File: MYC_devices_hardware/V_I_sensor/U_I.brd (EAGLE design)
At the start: 75.5 x 39.7 mm, 35 parts, among them IC2 MEGA8-AI, IC3 78L05, IC4 MAX3232CSE, Q1 20MH2, U1 INA219AIDCNR, X1 8-15V, X4 RS232

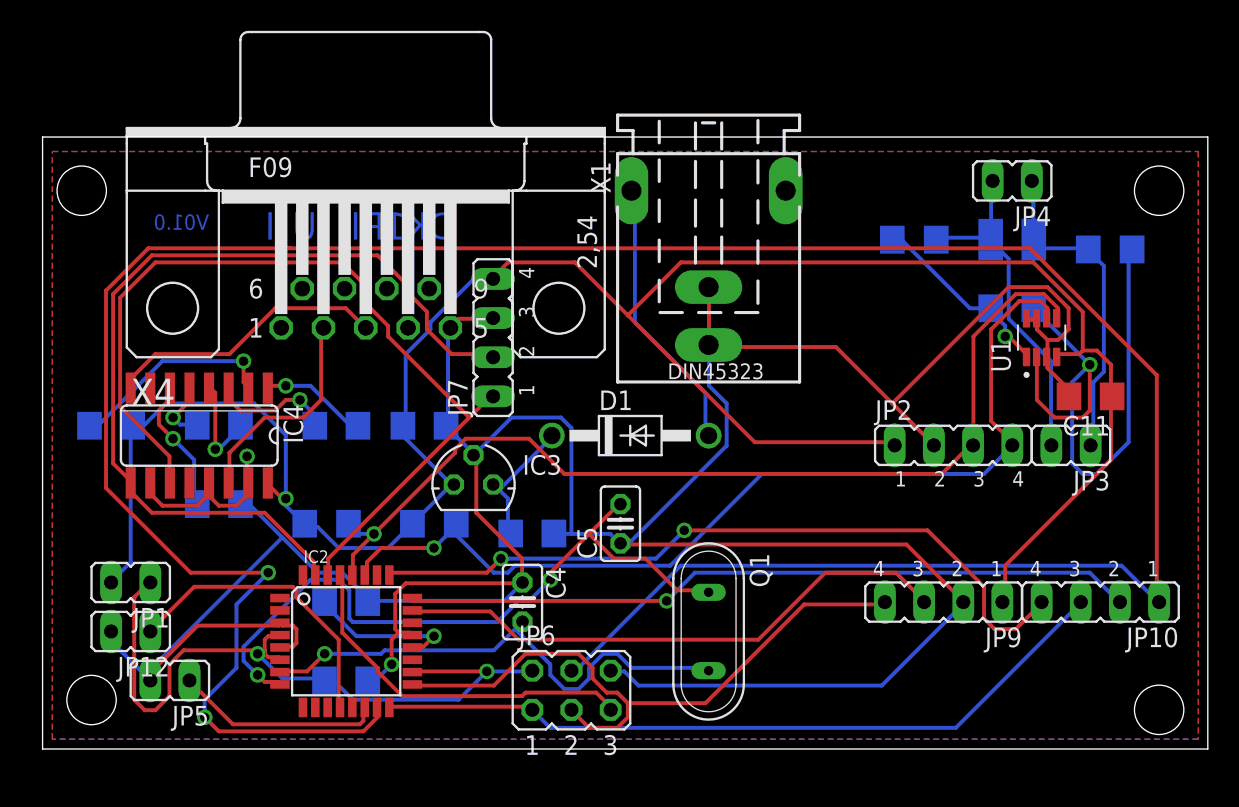
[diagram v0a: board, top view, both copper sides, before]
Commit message: reduced board!
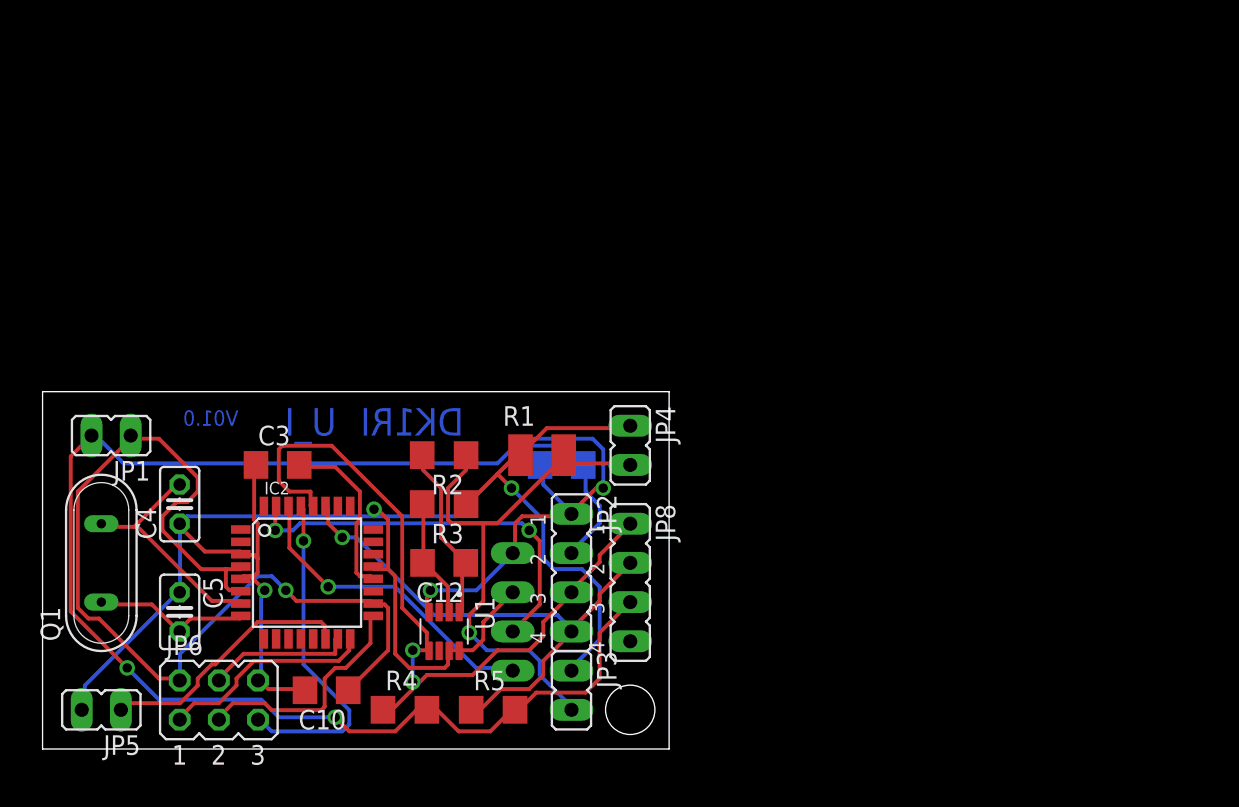
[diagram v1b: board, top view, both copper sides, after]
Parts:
- removed C1, C2: 22uF, rcl:C1206
- removed C6, C7, C8, C9: 220n, rcl:C1206
- removed D1: 1N4004, diode:DO41-10
- removed IC3: 78L05, v-reg:78LXX
- removed IC4: MAX3232CSE, maxim:SO16
- removed JP10, JP9: wireless, jumper:JP4
- removed JP12: no_remote, jumper:JP1
- removed X1: 8-15V, con-conrad:737992-5
- removed X4: RS232, con-subd:F09H
- added JP8: INA219, jumper:JP4
- R4, R5: value 10 -> 10k
- moved R3 46.2 mm to (26.0, 15.9), flipped to the top
- moved U1 43.2 mm to (26.0, 7.62), turned to 270 degrees
- moved C12 40.4 mm to (26.0, 12.1), flipped to the top
- moved Q1 39.6 mm to (3.81, 12.1), turned to 90 degrees
- moved JP3 36.1 mm to (34.3, 3.81), turned to 180 degrees
- moved C11 34.6 mm to (33.7, 18.4), flipped to the bottom
- moved R1 33.5 mm to (32.4, 19.1), flipped to the top
- moved R2 33.5 mm to (26.0, 19.1), flipped to the top, turned to 180 degrees
- moved JP4 30.1 mm to (38.1, 19.7), turned to 180 degrees
- moved C5 29.1 mm to (8.89, 8.89), turned to 270 degrees
- moved JP2 26.1 mm to (34.3, 11.4), turned to 270 degrees
- moved C4 23.1 mm to (8.89, 15.9), turned to 90 degrees
- moved JP6 22.9 mm to (11.4, 3.17)
- moved JP7 17.8 mm to (30.5, 8.89), flipped to the bottom
- moved R4 13.1 mm to (23.5, 2.54), flipped to the top
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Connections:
- removed net C13: C6.1, IC4.1
- removed net CLK0: IC2.25, JP10.4
- removed net GPIO1: IC2.24, JP10.2
- removed net N$10: IC4.14, X4.2
- removed net N$13: C7.1, IC4.4
- removed net N$14: C6.2, IC4.3
- removed net N$16: C8.1, IC4.2
- removed net N$17: C9.2, IC4.6
- removed net N$20: IC2.12, JP12.1
- removed net N$27: D1.A, X1.-1
- removed net N$3: C7.2, IC4.5
- removed net N$33: C1.1, D1.C, IC3.IN
- removed net N$41: IC4.8, X4.3
- removed net SCS: IC2.23, JP9.3
- net GND: no longer C1.2, C2.2, C9.1, IC3.GND, IC4.10, IC4.13, IC4.15, JP12.2, JP9.2, X1.+, X1.K, X4.5
- net N$12: no longer IC4.11
- net N$2: no longer IC4.9
- net N$22: now also JP8.1
- net N$26: no longer JP9.4
- net N$4: no longer JP10.3
- net N$5: now also JP8.2
- net N$9: no longer JP10.1
- net VDD: now also JP8.3; no longer C2.1, C8.2, IC3.OUT, IC4.16, JP9.1
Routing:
- net N$9: track 178.7 -> 9.43 mm, vias 2 -> 0
- net GND: track 237.2 -> 98.4 mm
- net CLK0: track 48.1 -> 0.00 mm, vias 2 -> 0
- net GPIO1: track 47.6 -> 0.00 mm, vias 1 -> 0
- net N$12: track 58.3 -> 20.5 mm, vias 0 -> 1
- net SCS: track 36.6 -> 0.00 mm
- net N$4: track 48.8 -> 14.0 mm
- net N$21: track 45.1 -> 10.4 mm, vias 2 -> 0
- net VDD: track 148.6 -> 116.2 mm, vias 1 -> 4
- net N$19: track 39.3 -> 7.80 mm, vias 1 -> 0
- net N$2: track 57.3 -> 26.0 mm, vias 0 -> 2
- net N$5: track 62.6 -> 35.2 mm
- net N$26: track 41.3 -> 15.3 mm
- net N$20: track 19.6 -> 0.00 mm
- net N$41: track 18.3 -> 0.00 mm
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- removed copper zone on layer 1, net GND
- removed copper zone on layer 16, net GND
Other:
- board size 75.5 x 39.7 mm -> 40.6 x 23.2 mm
